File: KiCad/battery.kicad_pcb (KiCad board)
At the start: 2 copper layers, 22.9 x 21.6 mm, 7 parts, among them J1 Conn_01x07_Male, J2 Conn_01x01_Male, J3 Conn_01x01_Male, U1 ATtiny85-20SU, U2 LD1117S33TR_SOT223

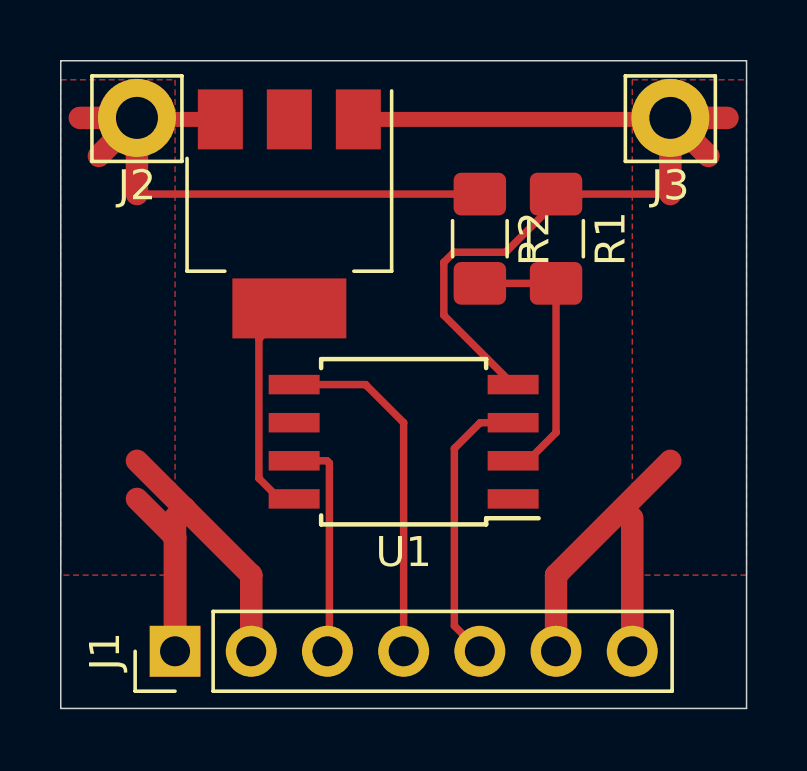
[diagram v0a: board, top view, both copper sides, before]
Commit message: better pcb
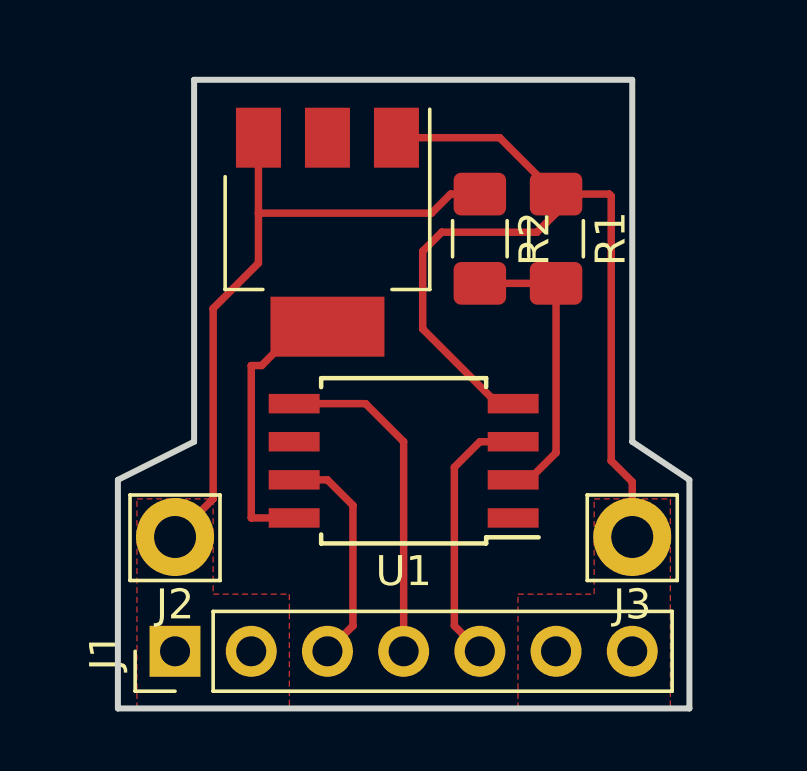
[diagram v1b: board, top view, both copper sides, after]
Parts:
- moved J3 14.0 mm to (151.1, 97.8)
- moved J2 14.0 mm to (135.9, 97.8)
- moved U2 1.41 mm to (141.0, 87.6)
- moved U1 0.64 mm to (143.5, 95.2)
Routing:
- net 12v: track 39.7 -> 22.1 mm
- net GND: track 42.6 -> 32.1 mm
- net 3.3v: track 7.54 -> 9.59 mm
- net VBatSensor: track 9.17 -> 9.99 mm
- net SDA: track 11.8 -> 11.2 mm
- net T: track 9.43 -> 8.80 mm
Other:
- board size 22.9 x 21.6 mm -> 19 x 21 mm
